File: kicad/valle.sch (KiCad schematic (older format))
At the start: 15 parts, among them IC1 ATMEGA8-P, IC2 L293D, P1 CONN_6, P2 CONN_6, P3 CONN_5X2

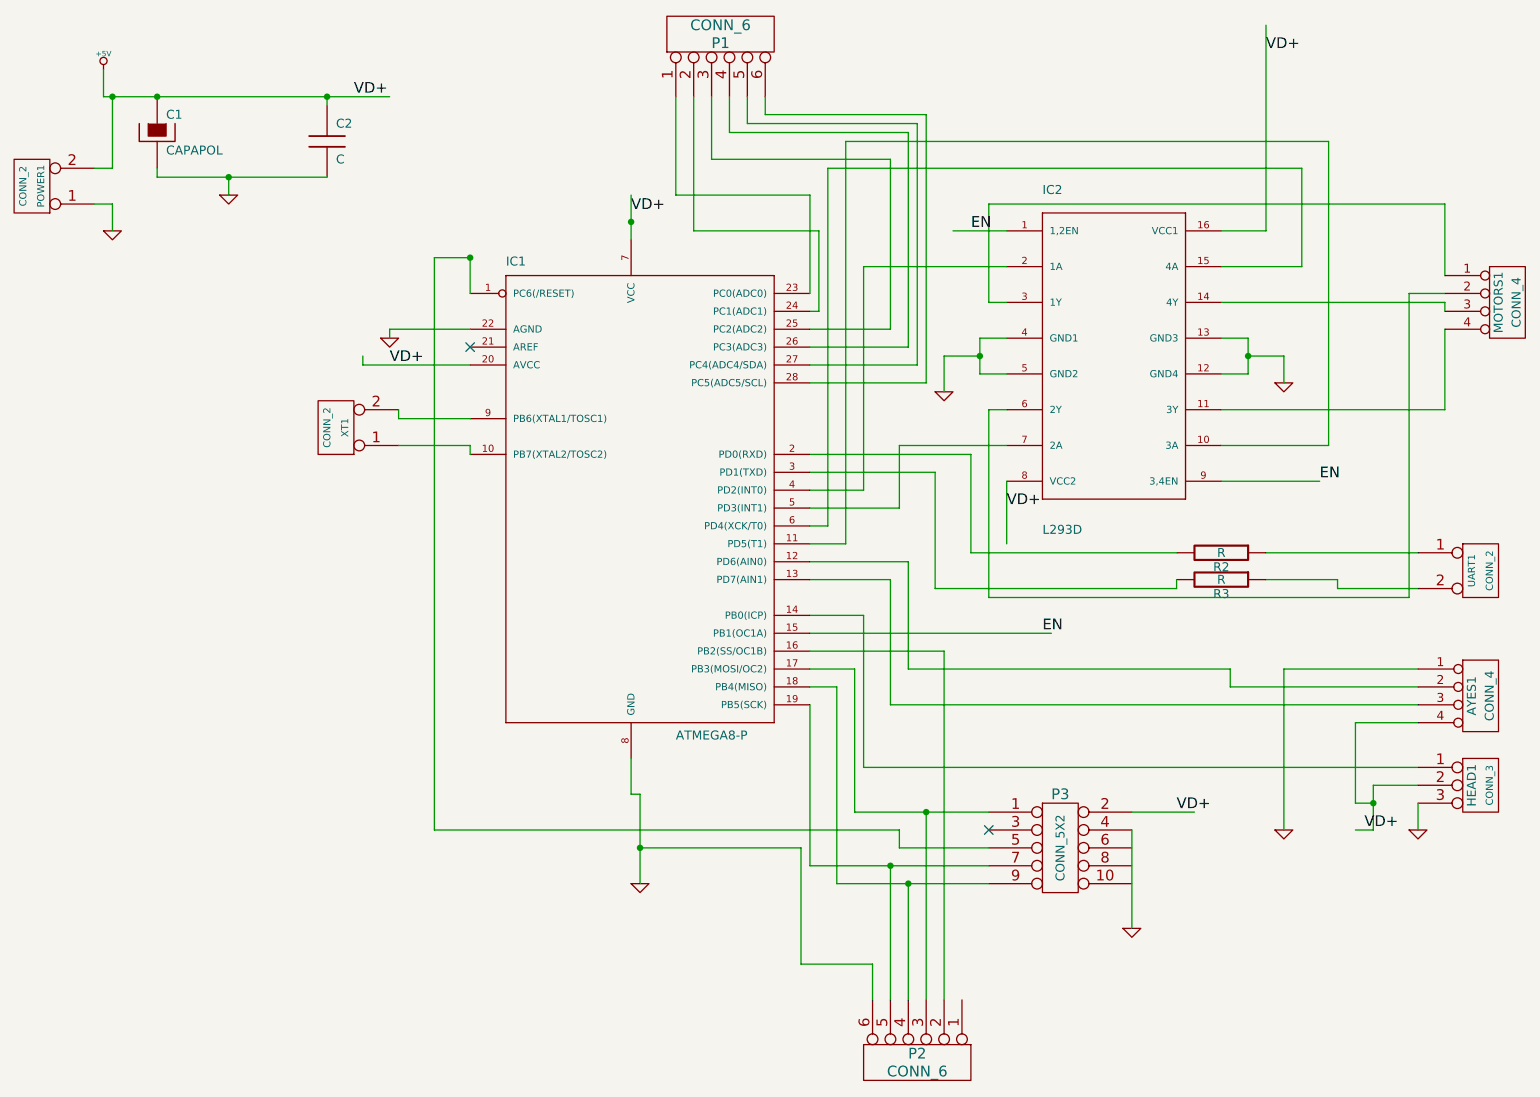
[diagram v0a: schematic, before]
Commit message: готовая плата
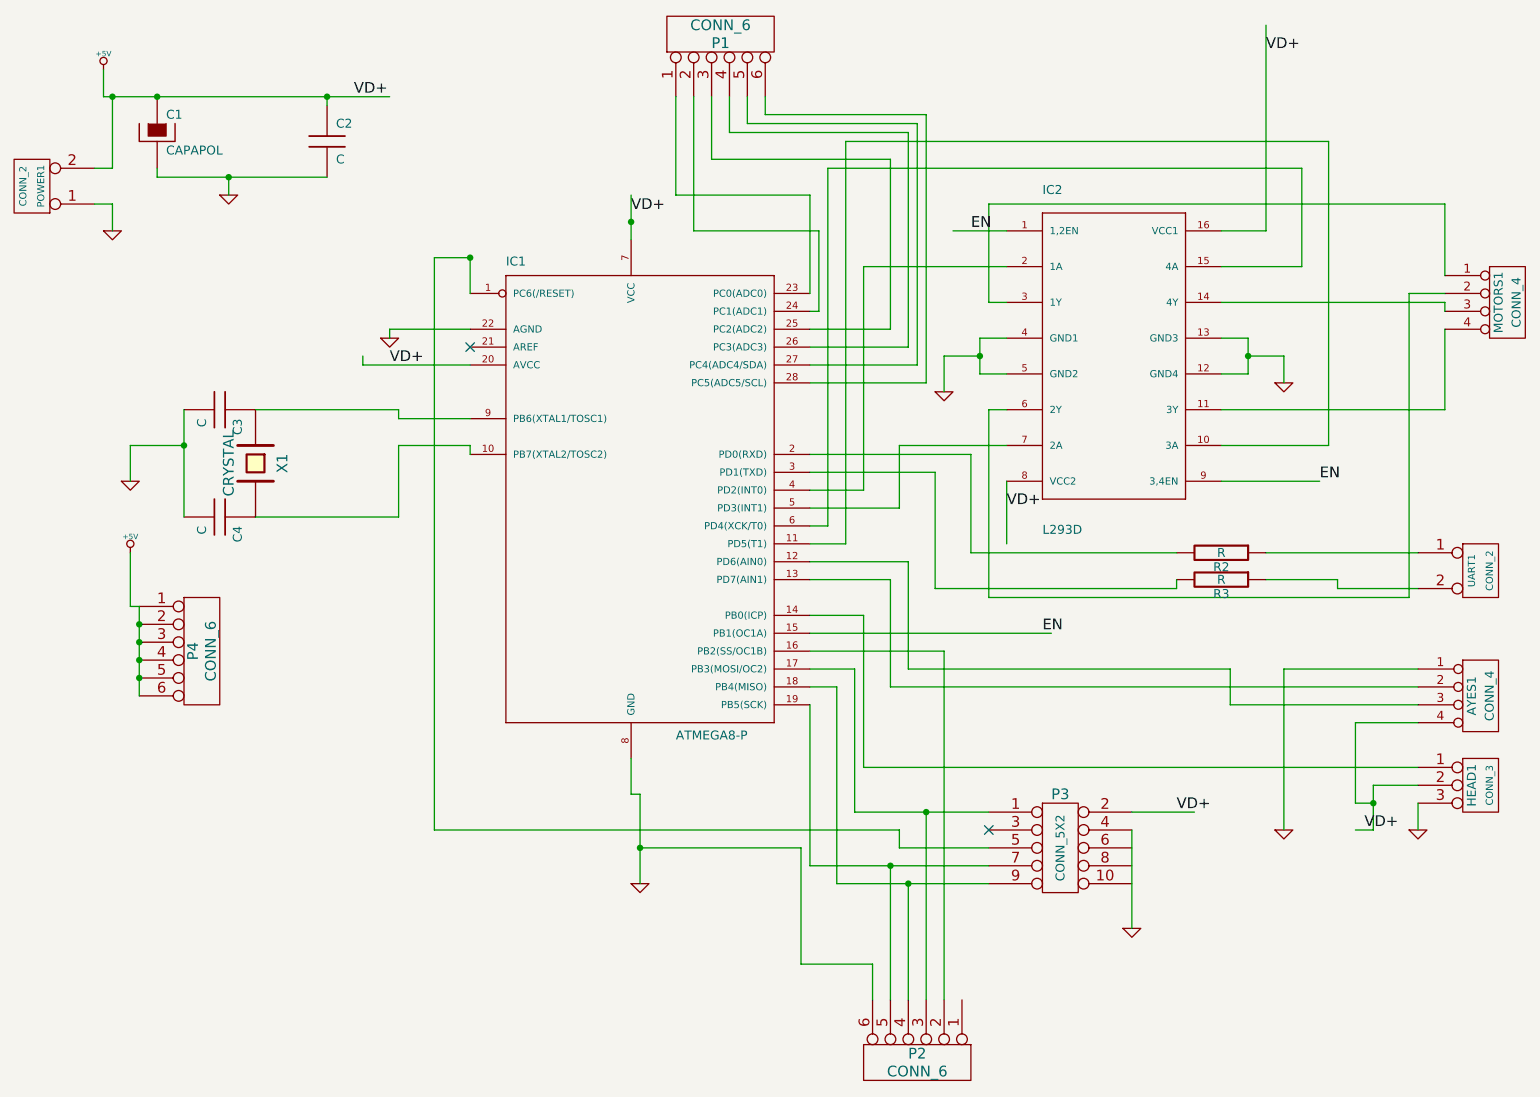
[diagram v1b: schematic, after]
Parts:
- removed XT1: CONN_2, symbol CONN_2
- added C3, C4: C, symbol C
- added P4: CONN_6, symbol CONN_6
- added X1: CRYSTAL, symbol CRYSTAL
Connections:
- wire segments 158 -> 155
